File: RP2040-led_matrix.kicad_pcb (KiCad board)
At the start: 2 copper layers, 187 parts, among them J2 USB_C_Receptacle, Q1 BSS84, Q10 BSS84, Q11 2N7002, Q12 2N7002, Q13 2N7002, Q14 2N7002, Q15 2N7002, Q16 2N7002, Q17 2N7002, Q18 2N7002, Q19 2N7002, Q2 BSS84, Q20 2N7002, Q3 BSS84, Q4 BSS84, Q5 BSS84, Q6 BSS84, Q7 BSS84, Q8 BSS84, Q9 BSS84, SW2 SW_DIP_x01, U1 W25Q16JVSS, U2 RP2040, U4 NCP1117-1.5_SOT223, Y2 ABM8-272-T3

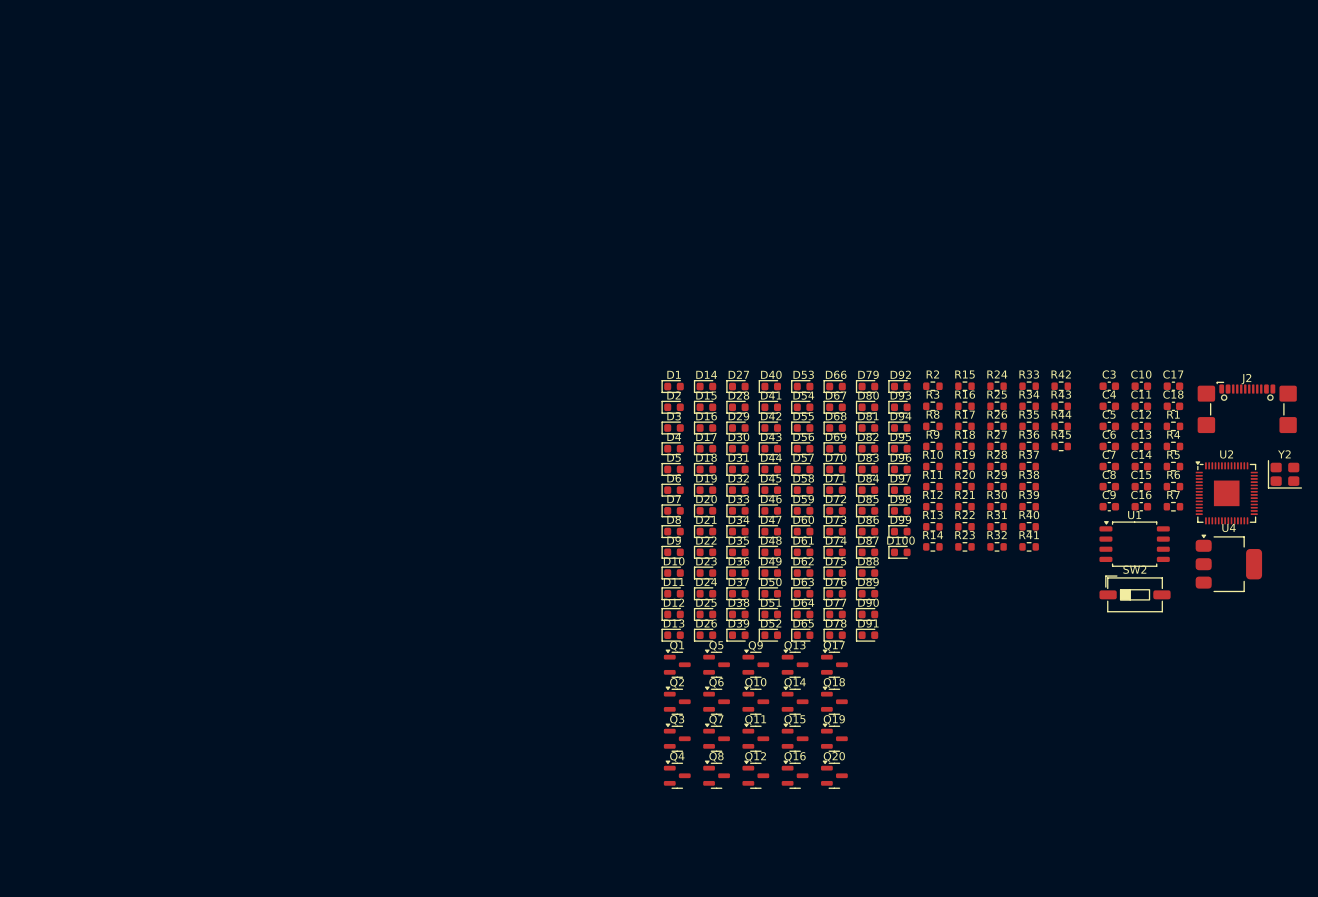
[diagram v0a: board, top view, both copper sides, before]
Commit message: improved design of the matrix
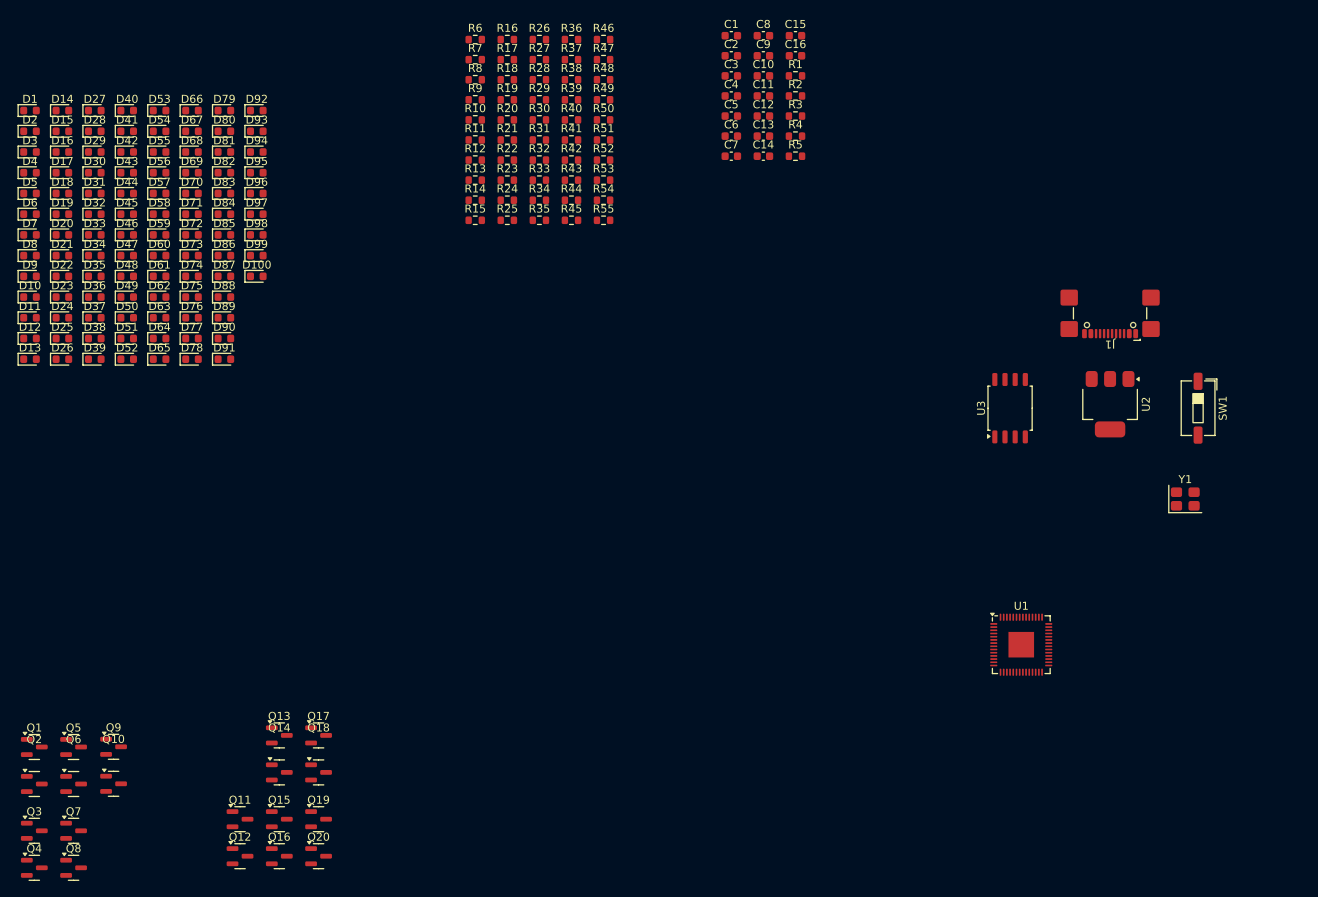
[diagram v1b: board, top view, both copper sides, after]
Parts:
- removed C17, C18: 100n, Capacitor_SMD:C_0603_1608Metric
- removed J2: USB_C_Receptacle, Connector_USB:USB_C_Receptacle_GCT_USB4110
- removed SW2: SW_DIP_x01, Button_Switch_SMD:SW_DIP_SPSTx01_Slide_6.7x4.1mm_W6.73mm_P2.54mm_LowProfile_JPin
- removed U4: NCP1117-1.5_SOT223, Package_TO_SOT_SMD:SOT-223-3_TabPin2
- removed Y2: ABM8-272-T3, Crystal:Crystal_SMD_3225-4Pin_3.2x2.5mm
- added C1: 15p, Capacitor_SMD:C_0603_1608Metric, F.Cu at (117.7, 16.4)
- added C2: 15p, Capacitor_SMD:C_0603_1608Metric, F.Cu at (117.7, 18.9)
- added J1: USB_C_Receptacle, Connector_USB:USB_C_Receptacle_GCT_USB4110, F.Cu at (165.0, 50.0)
- added R46: 100, Resistor_SMD:R_0603_1608Metric, F.Cu at (101.7, 16.9)
- added R47: 100, Resistor_SMD:R_0603_1608Metric, F.Cu at (101.7, 19.4)
- added R48: 100, Resistor_SMD:R_0603_1608Metric, F.Cu at (101.7, 21.9)
- added R49: 100, Resistor_SMD:R_0603_1608Metric, F.Cu at (101.7, 24.4)
- added R50: 100, Resistor_SMD:R_0603_1608Metric, F.Cu at (101.7, 27.0)
- added R51: 100, Resistor_SMD:R_0603_1608Metric, F.Cu at (101.7, 29.5)
- added R52: 100, Resistor_SMD:R_0603_1608Metric, F.Cu at (101.7, 32.0)
- added R53: 100, Resistor_SMD:R_0603_1608Metric, F.Cu at (101.7, 34.5)
- added R54: 100, Resistor_SMD:R_0603_1608Metric, F.Cu at (101.7, 37.0)
- added R55: 100, Resistor_SMD:R_0603_1608Metric, F.Cu at (101.7, 39.5)
- added SW1: SW_DIP_x01, Button_Switch_SMD:SW_DIP_SPSTx01_Slide_6.7x4.1mm_W6.73mm_P2.54mm_LowProfile_JPin, F.Cu at (176.0, 63.0)
- added U3: W25Q16JVSS, Package_SO:SOIC-8_5.3x5.3mm_P1.27mm, F.Cu at (152.5, 63.0)
- added Y1: ABM8-272-T3, Crystal:Crystal_SMD_3225-4Pin_3.2x2.5mm, F.Cu at (174.4, 74.3)
- C10, C9: value 10u -> 100n
- C13, C14, C15: value 100n -> 10u
- C3: value 1u -> 10u
- C4: value 1u -> 100n
- C6, C7: value 15p -> 100n
- R1: value 1k -> 5.1k
- R12, R18, R24, R33: value 100 -> 47
- R13, R19, R25, R28, R31, R34: value 100k -> 100
- R14, R20, R26, R29, R32, R36, R37, R40, R41, R44, R45, R8: value 100 -> 100k
- R15, R21, R27, R30, R9: value 100k -> 47
- R2: value 100 -> 5.1k
- R3: value 100k -> 1k
- R4: value 10k -> 1k
- R5: value 1k -> 100k
- R6: value 5.1k -> 47
- R7: value 5.1k -> 100
- U1: value W25Q16JVSS -> RP2040; footprint Package_SO:SOIC-8_5.3x5.3mm_P1.27mm -> Package_DFN_QFN:QFN-56-1EP_7x7mm_P0.4mm_EP3.2x3.2mm
- U2: value RP2040 -> NCP1117-1.5_SOT223; footprint Package_DFN_QFN:QFN-56-1EP_7x7mm_P0.4mm_EP3.2x3.2mm -> Package_TO_SOT_SMD:SOT-223-3_TabPin2
- moved R6 103.6 mm to (85.6, 16.9)
- moved R7 103.6 mm to (85.6, 19.4)
- moved D1 87.6 mm to (30.0, 25.8)
- moved D10 87.6 mm to (30.0, 49.1)
- moved D100 87.6 mm to (58.3, 46.5)
- moved D11 87.6 mm to (30.0, 51.7)
- moved D12 87.6 mm to (30.0, 54.3)
- moved D13 87.6 mm to (30.0, 56.9)
- moved D14 87.6 mm to (34.0, 25.8)
- moved D15 87.6 mm to (34.0, 28.4)
- moved D16 87.6 mm to (34.0, 31.0)
- moved D17 87.6 mm to (34.0, 33.6)
- moved D18 87.6 mm to (34.0, 36.2)
- moved D19 87.6 mm to (34.0, 38.7)
- moved D2 87.6 mm to (30.0, 28.4)
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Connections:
- C14 pad 1: +3.3V -> +5V
- C16 pad 1: +3.3V -> GND
- C16 pad 2: GND -> +3.3V
- C3 pad 1: +3.3V -> GND
- C3 pad 2: GND -> +1V1
- C6 pad 1: Net-(U2-XIN) -> +3.3V
- C7 pad 1: Net-(C7-Pad1) -> +3.3V
- C8 pad 1: GND -> +3.3V
- C8 pad 2: +3.3V -> GND
- C9 pad 1: +5V -> +3.3V
- Q1 pad 2: +5V -> Net-(Q1-S)
- Q10 pad 2: +5V -> Net-(Q10-S)
- Q2 pad 2: +5V -> Net-(Q2-S)
- Q3 pad 2: +5V -> Net-(Q3-S)
- Q4 pad 2: +5V -> Net-(Q4-S)
- Q5 pad 2: +5V -> Net-(Q5-S)
- Q6 pad 2: +5V -> Net-(Q6-S)
- Q7 pad 2: +5V -> Net-(Q7-S)
- Q8 pad 2: +5V -> Net-(Q8-S)
- Q9 pad 2: +5V -> Net-(Q9-S)
- R1 pad 2: /QSPI_SS -> GND
- R10 pad 1: C3 -> C2
- R10 pad 2: Net-(Q3-G) -> Net-(Q2-G)
- R11 pad 1: Net-(Q3-G) -> Net-(Q2-G)
- R11 pad 2: +5V -> Net-(Q2-S)
- R12 pad 1: R1 -> +3.3V
- R12 pad 2: Net-(Q11-G) -> Net-(Q3-S)
- R13 pad 1: Net-(Q11-G) -> C3
- R13 pad 2: GND -> Net-(Q3-G)
- R14 pad 1: C4 -> Net-(Q3-G)
- R14 pad 2: Net-(Q4-G) -> Net-(Q3-S)
- R15 pad 1: Net-(Q4-G) -> +3.3V
- R15 pad 2: +5V -> Net-(Q4-S)
- R16 pad 1: C5 -> C4
- R16 pad 2: Net-(Q5-G) -> Net-(Q4-G)
- R17 pad 1: Net-(Q5-G) -> Net-(Q4-G)
- R17 pad 2: +5V -> Net-(Q4-S)
- R18 pad 1: C6 -> +3.3V
- R18 pad 2: Net-(Q6-G) -> Net-(Q5-S)
- R19 pad 1: Net-(Q6-G) -> C5
- R19 pad 2: +5V -> Net-(Q5-G)
- R2 pad 1: C1 -> Net-(J1-CC2)
- R2 pad 2: Net-(Q1-G) -> GND
- R20 pad 1: C7 -> Net-(Q5-G)
- R20 pad 2: Net-(Q7-G) -> Net-(Q5-S)
- R21 pad 1: Net-(Q7-G) -> +3.3V
- R21 pad 2: +5V -> Net-(Q6-S)
- R22 pad 1: C8 -> C6
- R22 pad 2: Net-(Q8-G) -> Net-(Q6-G)
- R23 pad 1: Net-(Q8-G) -> Net-(Q6-G)
- R23 pad 2: +5V -> Net-(Q6-S)
- R24 pad 1: C9 -> +3.3V
- R24 pad 2: Net-(Q9-G) -> Net-(Q7-S)
- R25 pad 1: Net-(Q9-G) -> C7
- R25 pad 2: +5V -> Net-(Q7-G)
- R26 pad 1: C10 -> Net-(Q7-G)
- R26 pad 2: Net-(Q10-G) -> Net-(Q7-S)
- R27 pad 1: Net-(Q10-G) -> +3.3V
- R27 pad 2: +5V -> Net-(Q8-S)
- R28 pad 1: Net-(Q12-G) -> C8
- R28 pad 2: GND -> Net-(Q8-G)
- R29 pad 1: R2 -> Net-(Q8-G)
- R29 pad 2: Net-(Q12-G) -> Net-(Q8-S)
- R3 pad 1: Net-(Q1-G) -> Net-(U1-XOUT)
- R3 pad 2: +5V -> Net-(C2-Pad1)
- R30 pad 1: Net-(Q13-G) -> +3.3V
- R30 pad 2: GND -> Net-(Q9-S)
- R31 pad 1: Net-(Q14-G) -> C9
- R31 pad 2: GND -> Net-(Q9-G)
- R32 pad 1: R3 -> Net-(Q9-G)
- R32 pad 2: Net-(Q13-G) -> Net-(Q9-S)
- R33 pad 1: R4 -> +3.3V
- R33 pad 2: Net-(Q14-G) -> Net-(Q10-S)
- R34 pad 1: Net-(Q15-G) -> C10
- R34 pad 2: GND -> Net-(Q10-G)
- R35 pad 1: Net-(Q16-G) -> Net-(Q10-G)
- R35 pad 2: GND -> Net-(Q10-S)
- R36 pad 1: R5 -> Net-(Q11-G)
- R36 pad 2: Net-(Q15-G) -> GND
- R37 pad 1: R6 -> Net-(Q12-G)
- R37 pad 2: Net-(Q16-G) -> GND
- R38 pad 1: Net-(Q17-G) -> Net-(Q13-G)
- R39 pad 1: Net-(Q18-G) -> Net-(Q14-G)
- R4 pad 1: /QSPI_SS -> Net-(R4-Pad1)
- R4 pad 2: +3.3V -> /QSPI_SS
- R40 pad 1: R7 -> Net-(Q15-G)
- R40 pad 2: Net-(Q17-G) -> GND
- R41 pad 1: R8 -> Net-(Q16-G)
- R41 pad 2: Net-(Q18-G) -> GND
- R42 pad 1: Net-(Q19-G) -> Net-(Q17-G)
- R43 pad 1: Net-(Q20-G) -> Net-(Q18-G)
- R44 pad 1: R9 -> Net-(Q19-G)
- R44 pad 2: Net-(Q19-G) -> GND
- R45 pad 1: R10 -> Net-(Q20-G)
- R45 pad 2: Net-(Q20-G) -> GND
- R5 pad 1: Net-(U2-XOUT) -> /QSPI_SS
- R5 pad 2: Net-(C7-Pad1) -> +3.3V
- R6 pad 1: Net-(J2-CC1) -> +3.3V
- R6 pad 2: GND -> Net-(Q1-S)
- R7 pad 1: Net-(J2-CC2) -> C1
- R7 pad 2: GND -> Net-(Q1-G)
- R8 pad 1: C2 -> Net-(Q1-G)
- R8 pad 2: Net-(Q2-G) -> Net-(Q1-S)
- R9 pad 1: Net-(Q2-G) -> +3.3V
- R9 pad 2: +5V -> Net-(Q2-S)
- U1 pad 1: /QSPI_SS -> +3.3V
- U1 pad 2: /QSPI_SD1 -> unconnected-(U1-GPIO0-Pad2)
- U1 pad 3: /QSPI_SD2 -> C1
- U1 pad 4: GND -> C2
- U1 pad 5: /QSPI_SD0 -> C3
- U1 pad 6: /QSPI_SCLK -> C4
- U1 pad 7: /QSPI_SD3 -> C5
- U1 pad 8: +3.3V -> C6
- U2 pad 1: +3.3V -> GND
- U2 pad 2: unconnected-(U2-GPIO0-Pad2) -> +3.3V
- U2 pad 3: C1 -> +5V
